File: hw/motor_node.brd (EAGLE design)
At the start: 27.6 x 27.3 mm, 55 parts, among them IC1 TINY84 or TINY841, IC3 MCP1703DB, Q1 BSS138, Q2 BSS138, Q3 BSS138

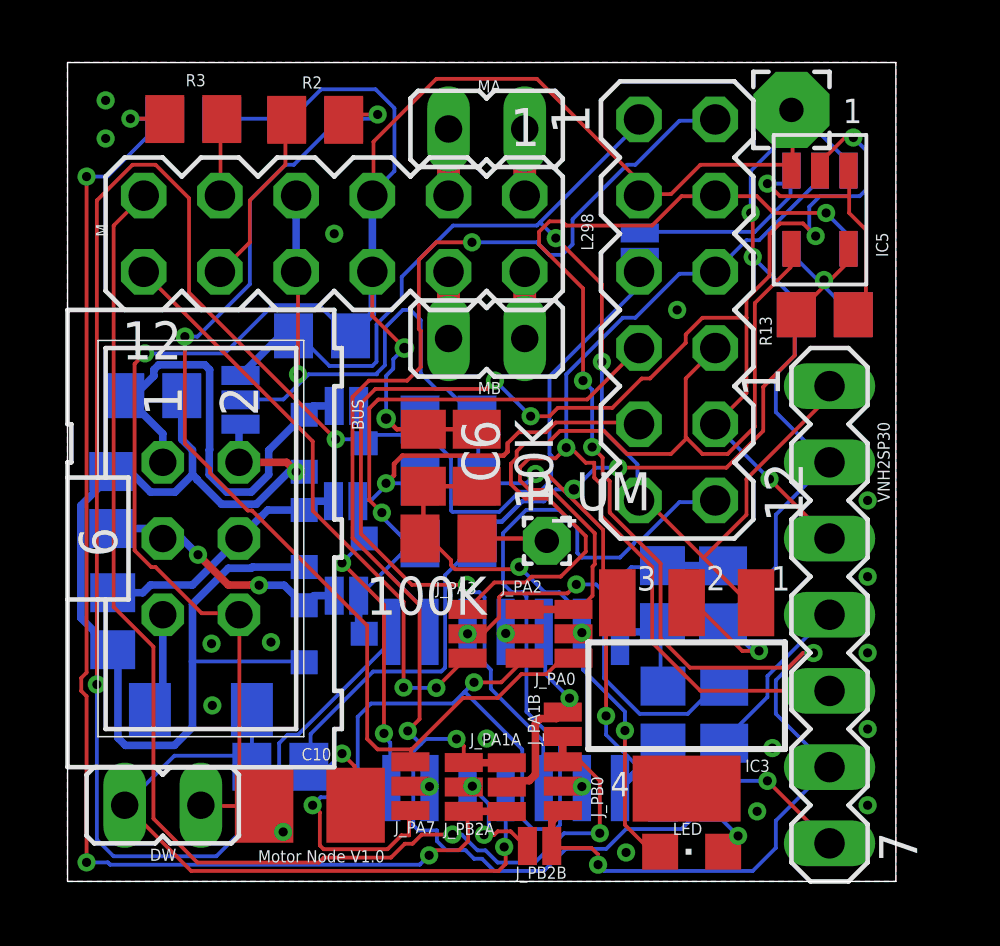
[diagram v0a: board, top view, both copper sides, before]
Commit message: some files updated
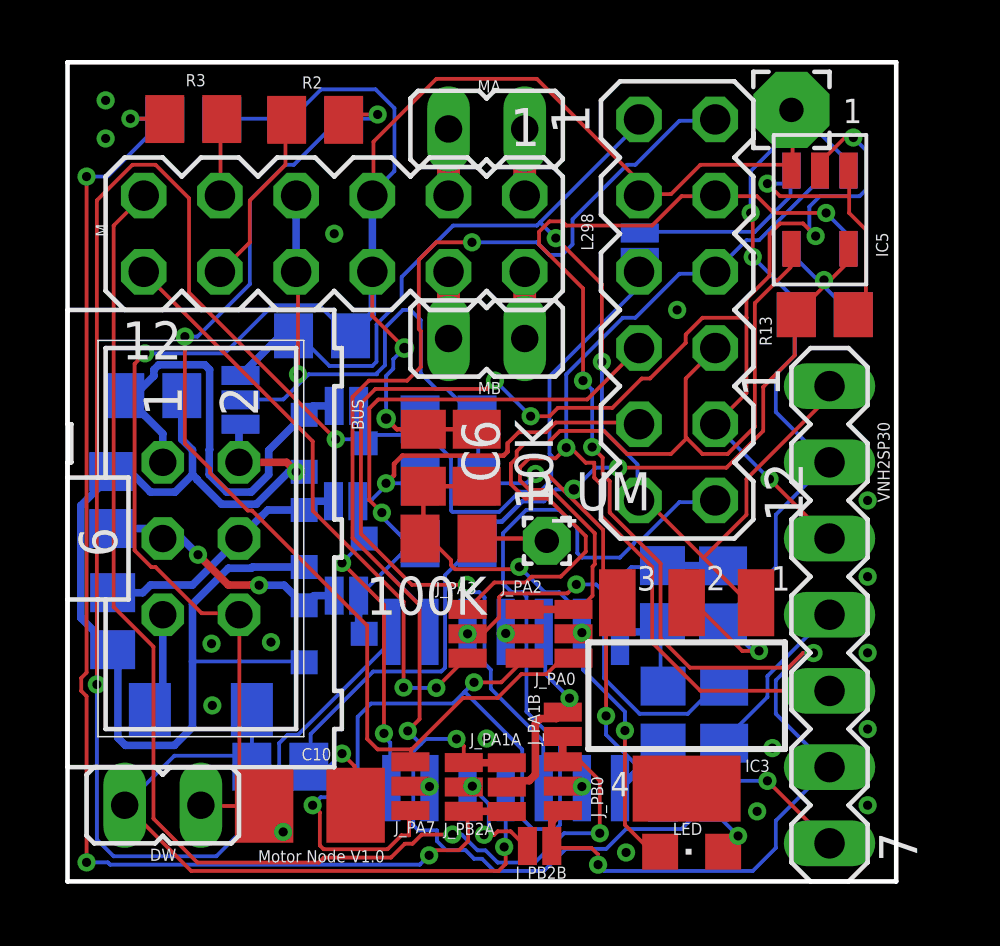
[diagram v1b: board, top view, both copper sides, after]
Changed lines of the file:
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@@
 <setting verticaltext="up"/>
 </settings>
-<grid distance="25" unitdist="mil" unit="mil" style="dots" multiple="1" display="yes" altdistance="1" altunitdist="mil" altunit="mil"/>
+<grid distance="12.5" unitdist="mil" unit="mil" style="dots" multiple="2" display="yes" altdistance="1" altunitdist="mil" altunit="mil"/>
 <layers>
 <layer number="1" name="Top" color="4" fill="1" visible="yes" active="yes"/>
@@
 <wire x1="0" y1="27.295" x2="0" y2="0" width="0" layer="20"/>
 <text x="6.35" y="0.635" size="0.4064" layer="25">Motor Node V1.0</text>
+<wire x1="0" y1="0" x2="27.6225" y2="0" width="0.1524" layer="20"/>
+<wire x1="27.6225" y1="0" x2="27.6225" y2="27.305" width="0.1524" layer="20"/>
+<wire x1="27.6225" y1="27.305" x2="0" y2="27.305" width="0.1524" layer="20"/>
+<wire x1="0" y1="27.305" x2="0" y2="0" width="0.1524" layer="20"/>
 </plain>
 <attributes>
